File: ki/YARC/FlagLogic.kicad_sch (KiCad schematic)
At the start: 11 parts, among them U105 74LS86, U106 74LS139, U107 74HC00, U108 74HC02, U109 74LS32, U110 74LS21, U111 74LS153, U112 74LS573, U113 74LS573, U114 74LS574, U115 74LS574

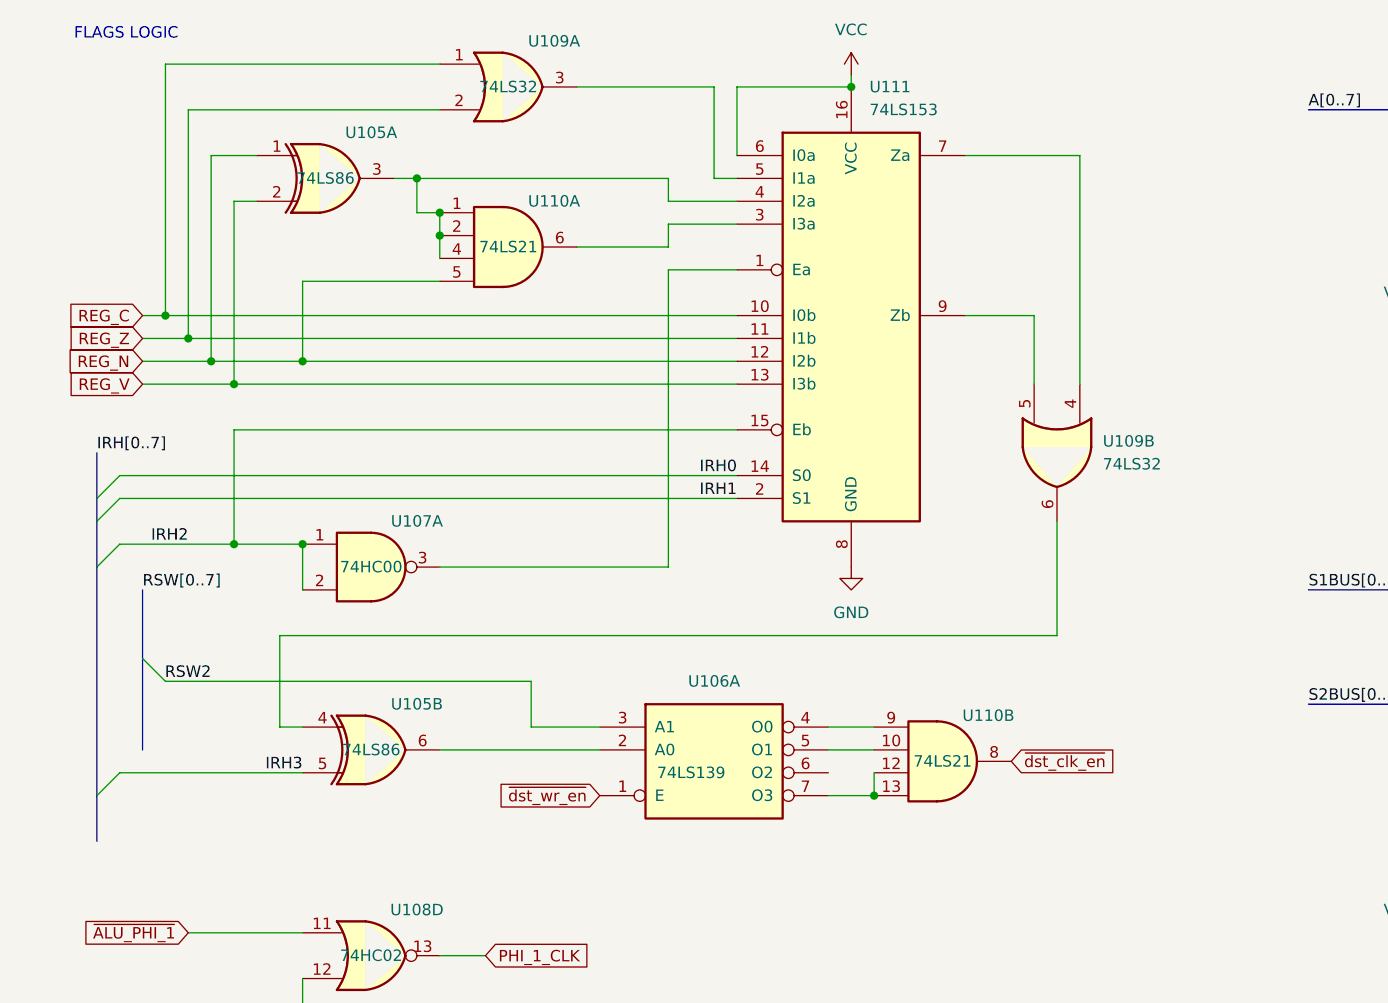
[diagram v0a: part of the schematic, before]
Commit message: Believable ALU/Flags design almost complete
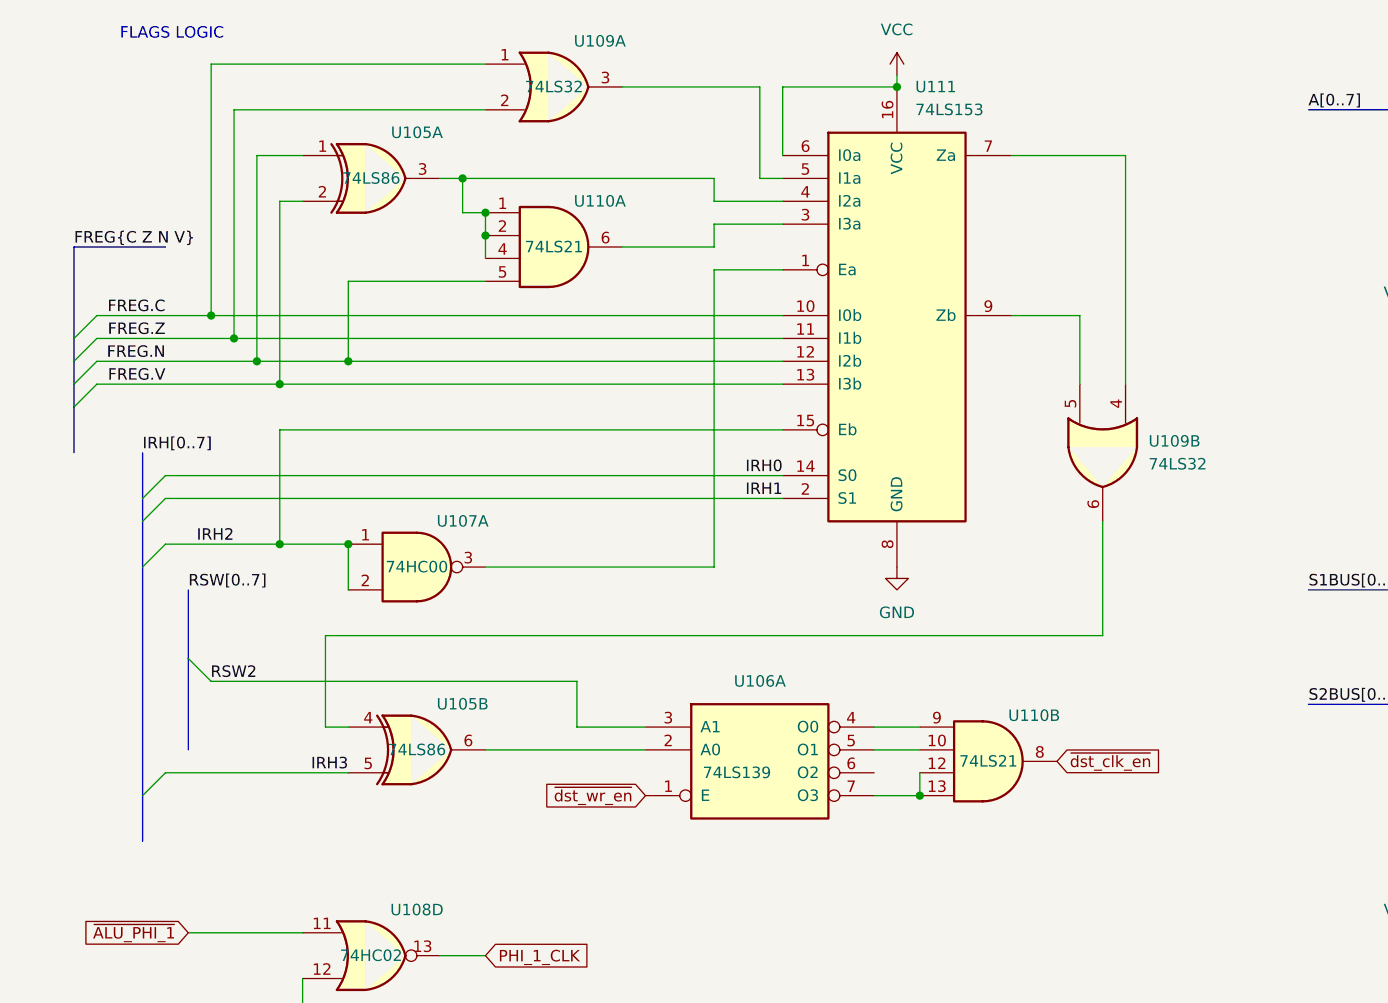
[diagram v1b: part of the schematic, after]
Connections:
- net REG_C renamed FREG.C
- net REG_N renamed FREG.N
- net REG_V renamed FREG.V
- net REG_Z renamed FREG.Z
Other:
- moved on the sheet: U105A, U105B, U106A, U107A, U109A, U109B, U110A, U110B, U111
